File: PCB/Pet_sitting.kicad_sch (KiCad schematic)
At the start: 15 parts, among them IC1 ESP32-CAM, J1 Conn_01x02, J2 Conn_01x02_Female, J3 Conn_01x02, J4 Conn_01x02, J5 Conn_01x06_Female, M1 Motor_Servo, U1 DFR0299, U2 L293D, U3 LM1117-5.0

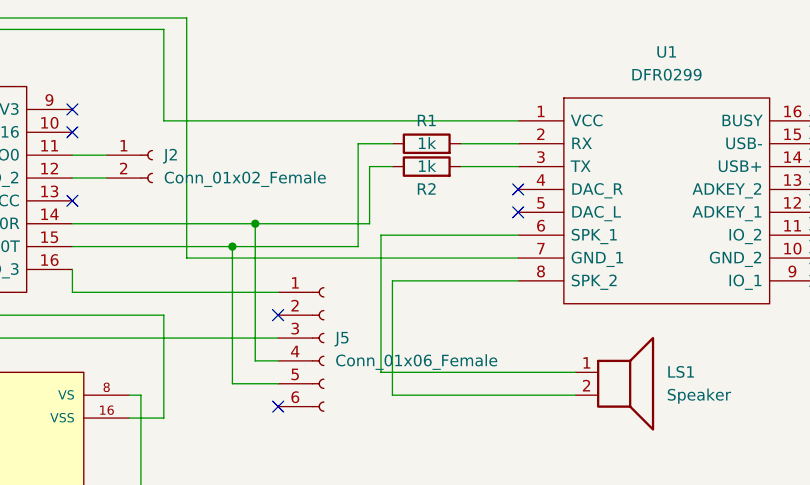
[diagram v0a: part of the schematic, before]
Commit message: Add files via upload
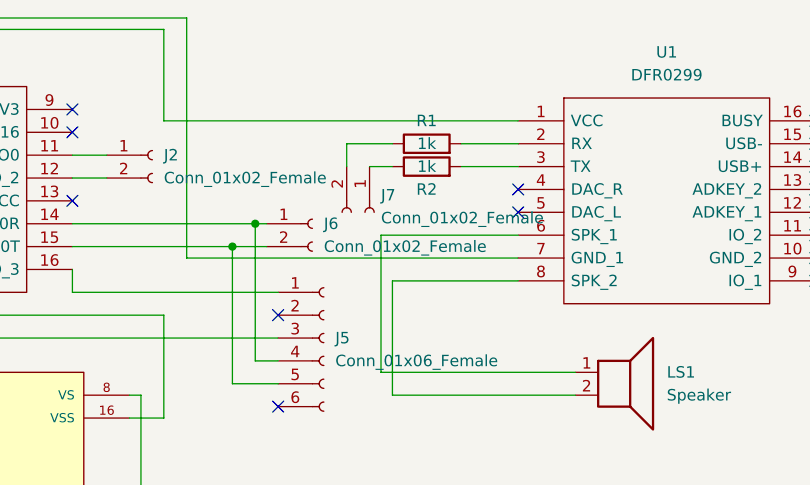
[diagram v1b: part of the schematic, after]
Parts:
- added J6, J7: Conn_01x02_Female, Connector_PinSocket_2.54mm:PinSocket_1x02_P2.54mm_Vertical, symbol Connector:Conn_01x02_Female
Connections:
- net at IC1.14 (U0R), J5.4 (Pin_4): now also J6.1 (Pin_1); no longer R2.1
- net at IC1.15 (U0T), J5.5 (Pin_5): now also J6.2 (Pin_2); no longer R1.1
- new net: J7.1 (Pin_1), R2.1
- new net: J7.2 (Pin_2), R1.1
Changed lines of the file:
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@@
   (junction (at 111.76 77.47) (diameter 0) (color 0 0 0 0)
   )
+  (junction (at 175.26 85.09) (diameter 0) (color 0 0 0 0)
+  )
   (junction (at 124.46 69.85) (diameter 0) (color 0 0 0 0)
   )
   (junction (at 177.8 82.55) (diameter 0) (color 0 0 0 0)
-  )
-  (junction (at 175.26 85.09) (diameter 0) (color 0 0 0 0)
   )
   (no_connect (at 127 87.63))
@@
     (stroke (width 0) (type default) (color 0 0 0 0))
   )
+  (wire (pts (xy 190.5 76.2) (xy 193.04 76.2))
+    (stroke (width 0) (type default) (color 0 0 0 0))
+  )
   (wire (pts (xy 165.1 142.24) (xy 74.93 142.24))
     (stroke (width 0) (type default) (color 0 0 0 0))
@@
     (stroke (width 0) (type default) (color 0 0 0 0))
   )
-  (wire (pts (xy 193.04 76.2) (xy 190.5 76.2))
-    (stroke (width 0) (type default) (color 0 0 0 0))
-  )
   (wire (pts (xy 207.01 71.12) (xy 167.64 71.12))
     (stroke (width 0) (type default) (color 0 0 0 0))
@@
     (stroke (width 0) (type default) (color 0 0 0 0))
   )
-  (wire (pts (xy 189.23 73.66) (xy 189.23 85.09))
-    (stroke (width 0) (type default) (color 0 0 0 0))
-  )
   (wire (pts (xy 163.83 124.46) (xy 172.72 124.46))
     (stroke (width 0) (type default) (color 0 0 0 0))
@@
     (stroke (width 0) (type default) (color 0 0 0 0))
   )
-  (wire (pts (xy 193.04 73.66) (xy 189.23 73.66))
-    (stroke (width 0) (type default) (color 0 0 0 0))
-  )
   (wire (pts (xy 163.83 101.6) (xy 165.1 101.6))
     (stroke (width 0) (type default) (color 0 0 0 0))
@@
     (stroke (width 0) (type default) (color 0 0 0 0))
   )
-  (wire (pts (xy 175.26 85.09) (xy 189.23 85.09))
-    (stroke (width 0) (type default) (color 0 0 0 0))
-  )
   (wire (pts (xy 72.39 72.39) (xy 71.12 72.39))
     (stroke (width 0) (type default) (color 0 0 0 0))
@@
     (stroke (width 0) (type default) (color 0 0 0 0))
   )
-  (wire (pts (xy 190.5 82.55) (xy 177.8 82.55))
-    (stroke (width 0) (type default) (color 0 0 0 0))
-  )
   (wire (pts (xy 154.94 144.78) (xy 72.39 144.78))
     (stroke (width 0) (type default) (color 0 0 0 0))
@@
     (stroke (width 0) (type default) (color 0 0 0 0))
   )
+  (wire (pts (xy 177.8 82.55) (xy 179.07 82.55))
+    (stroke (width 0) (type default) (color 0 0 0 0))
+  )
   (wire (pts (xy 74.93 142.24) (xy 74.93 69.85))
     (stroke (width 0) (type default) (color 0 0 0 0))
@@
     (stroke (width 0) (type default) (color 0 0 0 0))
   )
+  (wire (pts (xy 175.26 85.09) (xy 179.07 85.09))
+    (stroke (width 0) (type default) (color 0 0 0 0))
+  )
   (wire (pts (xy 116.84 69.85) (xy 116.84 83.82))
     (stroke (width 0) (type default) (color 0 0 0 0))
@@
     (stroke (width 0) (type default) (color 0 0 0 0))
   )
-  (wire (pts (xy 190.5 76.2) (xy 190.5 82.55))
-    (stroke (width 0) (type default) (color 0 0 0 0))
-  )
   (wire (pts (xy 114.3 82.55) (xy 81.28 82.55))
     (stroke (width 0) (type default) (color 0 0 0 0))
@@
     (stroke (width 0) (type default) (color 0 0 0 0))
   )
+  (wire (pts (xy 187.96 73.66) (xy 187.96 76.2))
+    (stroke (width 0) (type default) (color 0 0 0 0))
+  )
   (wire (pts (xy 167.64 104.14) (xy 163.83 104.14))
     (stroke (width 0) (type default) (color 0 0 0 0))
@@
   )
   (wire (pts (xy 119.38 116.84) (xy 119.38 77.47))
+    (stroke (width 0) (type default) (color 0 0 0 0))
+  )
+  (wire (pts (xy 193.04 73.66) (xy 187.96 73.66))
     (stroke (width 0) (type default) (color 0 0 0 0))
   )
@@
     (pin "1")
   )
+  (symbol (lib_id "Connector:Conn_01x02_Female") (at 190.5 81.28 270) (unit 1)
+    (in_bom yes) (on_board yes) (fields_autoplaced)
+    (property "Reference" "J7" (id 0) (at 191.77 79.3749 90)
+      (effects (font (size 1.27 1.27)) (justify left))
+    )
+    (property "Value" "Conn_01x02_Female" (id 1) (at 191.77 81.9149 90)
+      (effects (font (size 1.27 1.27)) (justify left))
+    )
+    (property "Footprint" "Connector_PinSocket_2.54mm:PinSocket_1x02_P2.54mm_Vertical" (id 2) (at 190.5 81.28 0)
+      (effects (font (size 1.27 1.27)) hide)
+    )
+    (property "Datasheet" "~" (id 3) (at 190.5 81.28 0)
+      (effects (font (size 1.27 1.27)) hide)
+    )
+    (pin "1")
+    (pin "2")
+  )
   (symbol (lib_id "Regulator_Linear:LM1117-5.0") (at 91.44 69.85 0) (unit 1)
     (in_bom yes) (on_board yes) (fields_autoplaced)
@@
     (pin "2")
   )
+  (symbol (lib_id "Connector:Conn_01x02_Female") (at 184.15 82.55 0) (unit 1)
+    (in_bom yes) (on_board yes) (fields_autoplaced)
+    (property "Reference" "J6" (id 0) (at 185.42 82.5499 0)
+      (effects (font (size 1.27 1.27)) (justify left))
+    )
+    (property "Value" "Conn_01x02_Female" (id 1) (at 185.42 85.0899 0)
+      (effects (font (size 1.27 1.27)) (justify left))
+    )
+    (property "Footprint" "Connector_PinSocket_2.54mm:PinSocket_1x02_P2.54mm_Vertical" (id 2) (at 184.15 82.55 0)
+      (effects (font (size 1.27 1.27)) hide)
+    )
+    (property "Datasheet" "~" (id 3) (at 184.15 82.55 0)
+      (effects (font (size 1.27 1.27)) hide)
+    )
+    (pin "1")
+    (pin "2")
+  )
   (symbol (lib_id "Device:R") (at 196.85 73.66 90) (unit 1)
     (in_bom yes) (on_board yes)
@@
       (reference "J5") (unit 1) (value "Conn_01x06_Female") (footprint "Connector_PinSocket_2.54mm:PinSocket_1x06_P2.54mm_Vertical")
     )
+    (path "/b19f0701-c82d-49f1-9572-fc8213276e5f"
+      (reference "J6") (unit 1) (value "Conn_01x02_Female") (footprint "Connector_PinSocket_2.54mm:PinSocket_1x02_P2.54mm_Vertical")
+    )
+    (path "/2166914e-d063-4fa4-be83-66e3b9e42f94"
+      (reference "J7") (unit 1) (value "Conn_01x02_Female") (footprint "Connector_PinSocket_2.54mm:PinSocket_1x02_P2.54mm_Vertical")
+    )
     (path "/5921a3a8-198b-4bd9-8309-8da619455916"
